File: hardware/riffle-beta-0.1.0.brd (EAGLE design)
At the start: 102.6 x 18.2 mm, 49 parts, among them IC1 ATMEGA328P, IC2 MCP73831, IC3 CH340G, IC5 24AA128SN, IC7 MIC5225-3.3V, IC8 MIC5225-3.3V, J1 AYZ0202, X2 12MHz, X3 16 MHz

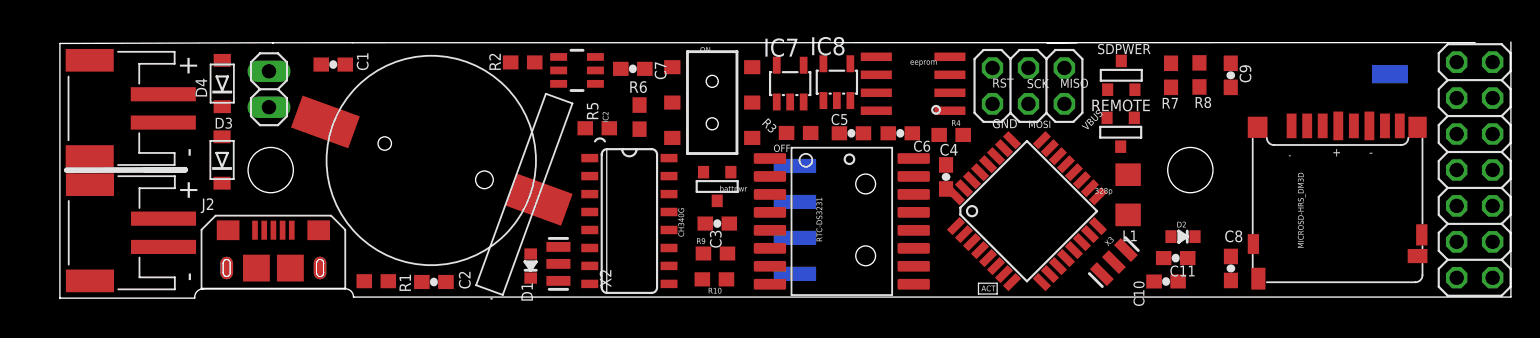
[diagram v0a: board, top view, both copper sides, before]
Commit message: update
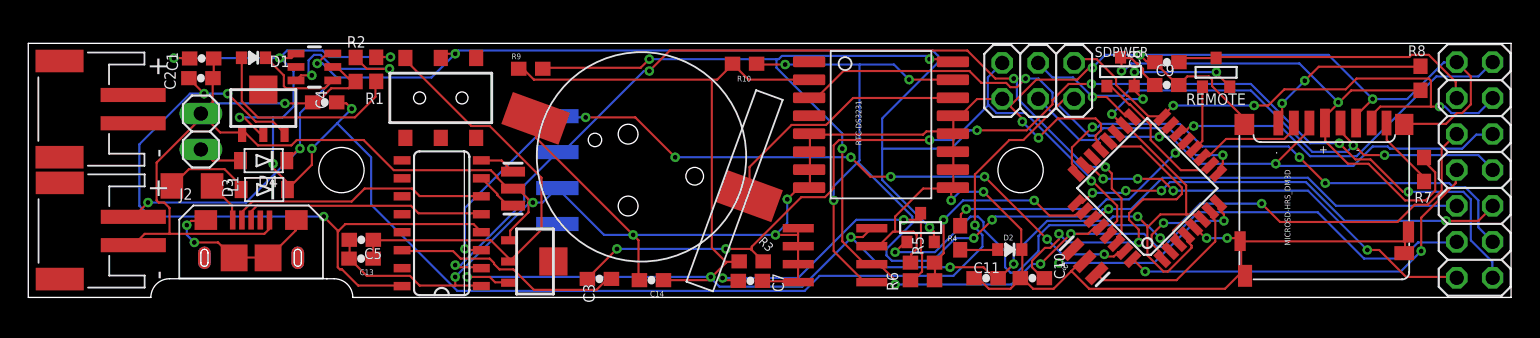
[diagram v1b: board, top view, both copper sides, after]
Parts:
- removed C6: 10uF, SparkFun:0603-CAP
- removed IC7, IC8: MIC5225-3.3V, adafruit:SOT23-5L
- removed RTC: (no value), wirepad:SMD1,27-2,54
- added C13, C14: 10uF, SparkFun:0603-CAP
- added IC4, IC6: MCP1700-33, adafruit:SOT89
- R7, R8: value 50K -> 10K
- moved L1 66.2 mm to (9.43, 7.88), turned to 180 degrees
- moved C4 44.2 mm to (18.8, 13.8), turned to 180 degrees
- moved C5 35.4 mm to (21.4, 4.07), turned to 180 degrees
- moved R5 24.9 mm to (61.1, 2.46)
- moved D1 24.5 mm to (13.8, 16.9), turned to 180 degrees
- moved R6 23.1 mm to (61.1, 1.22), turned to 180 degrees
- moved C2 21.9 mm to (10.1, 15.5), turned to 0 degrees
- moved J1 19.2 mm to (27.0, 14.1), turned to 0 degrees
- moved R7 19.1 mm to (96.5, 9.05)
- moved IC2 18.6 mm to (18.1, 16.3), turned to 90 degrees
- moved R9 18.5 mm to (33.4, 16.2)
- moved JP3 17.2 mm to (40.3, 9.00)
- moved C7 17.1 mm to (48.9, 1.17)
- moved R8 15.6 mm to (96.3, 15.5), turned to 270 degrees
- moved R10 15.4 mm to (48.5, 16.5)
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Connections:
- removed net D5: IC1.9, JP3.4
- removed net N$12: RTC-DS3231.3, RTC.1
- new net D5/RST: JP3.4
- new net D5/RTC: IC1.9, RTC-DS3231.3
- net A1: now also JP5.12; no longer JP3.1
- net A2: now also JP5.10; no longer JP3.2
- net GND: now also C13.2, C14.2, IC4.1, IC6.1; no longer C6.2, IC7.2, IC8.2
- net N$8: now also IC6.3; no longer IC7.5
- net RXD: now also JP3.2; no longer JP5.10
- net TXD: now also JP3.1; no longer JP5.12
- net VBUS: now also IC6.2; no longer IC7.1, IC7.3
- net VCC: now also C14.1, IC4.3; no longer C6.1, IC8.5
- net VDD: now also C13.1, IC4.2; no longer IC8.1, IC8.3
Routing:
- net GND: track 0.00 -> 296.5 mm, vias 0 -> 15
- net VBAT: track 0.00 -> 138.5 mm, vias 0 -> 9
- net VCC: track 0.00 -> 132.9 mm, vias 0 -> 10
- net VBUS: track 0.00 -> 112.2 mm, vias 0 -> 8
- net SCL: track 0.00 -> 96.2 mm, vias 0 -> 6
- net SDA: track 0.00 -> 86.0 mm, vias 0 -> 6
- net RXD: track 0.00 -> 64.9 mm, vias 0 -> 4
- net TXD: track 0.00 -> 57.8 mm, vias 0 -> 8
- net RESET: track 0.00 -> 54.4 mm, vias 0 -> 4
- net N$8: track 0.00 -> 51.8 mm, vias 0 -> 3
- net N$4: track 0.00 -> 42.8 mm, vias 0 -> 2
- net SCK: track 0.00 -> 41.5 mm, vias 0 -> 3
- net MISO: track 0.00 -> 40.4 mm, vias 0 -> 3
- net MOSI: track 0.00 -> 40.3 mm, vias 0 -> 2
- net A1: track 0.00 -> 36.9 mm, vias 0 -> 3
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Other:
- board size 102.6 x 18.2 mm -> 104.8 x 18 mm
- board text removed: "328p"
- board text removed: "ACT"
- board text removed: "CH340G"
- board text removed: "D5"
- board text removed: "GND"
- board text removed: "IC2"
- board text removed: "MISO"
- board text removed: "MOSI"
- board text removed: "OFF"
- board text removed: "ON"
- board text removed: "RIFFLE-328p ver 0.95"
- board text removed: "RST"
- board text removed: "SCK"
- board text removed: "VBUS"
- board text removed: "X2"
- board text removed: "all dimensions in mm"
- board text removed: "battpwr"
- board text removed: "eeprom"
- board text removed: "publiclab.org/wiki/riffle"
